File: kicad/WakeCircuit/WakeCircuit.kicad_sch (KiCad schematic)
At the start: 15 parts, among them J1 Conn_01x12_Socket, J2 Conn_01x10_Socket, U1 TLV7011DBVR, U3 4013

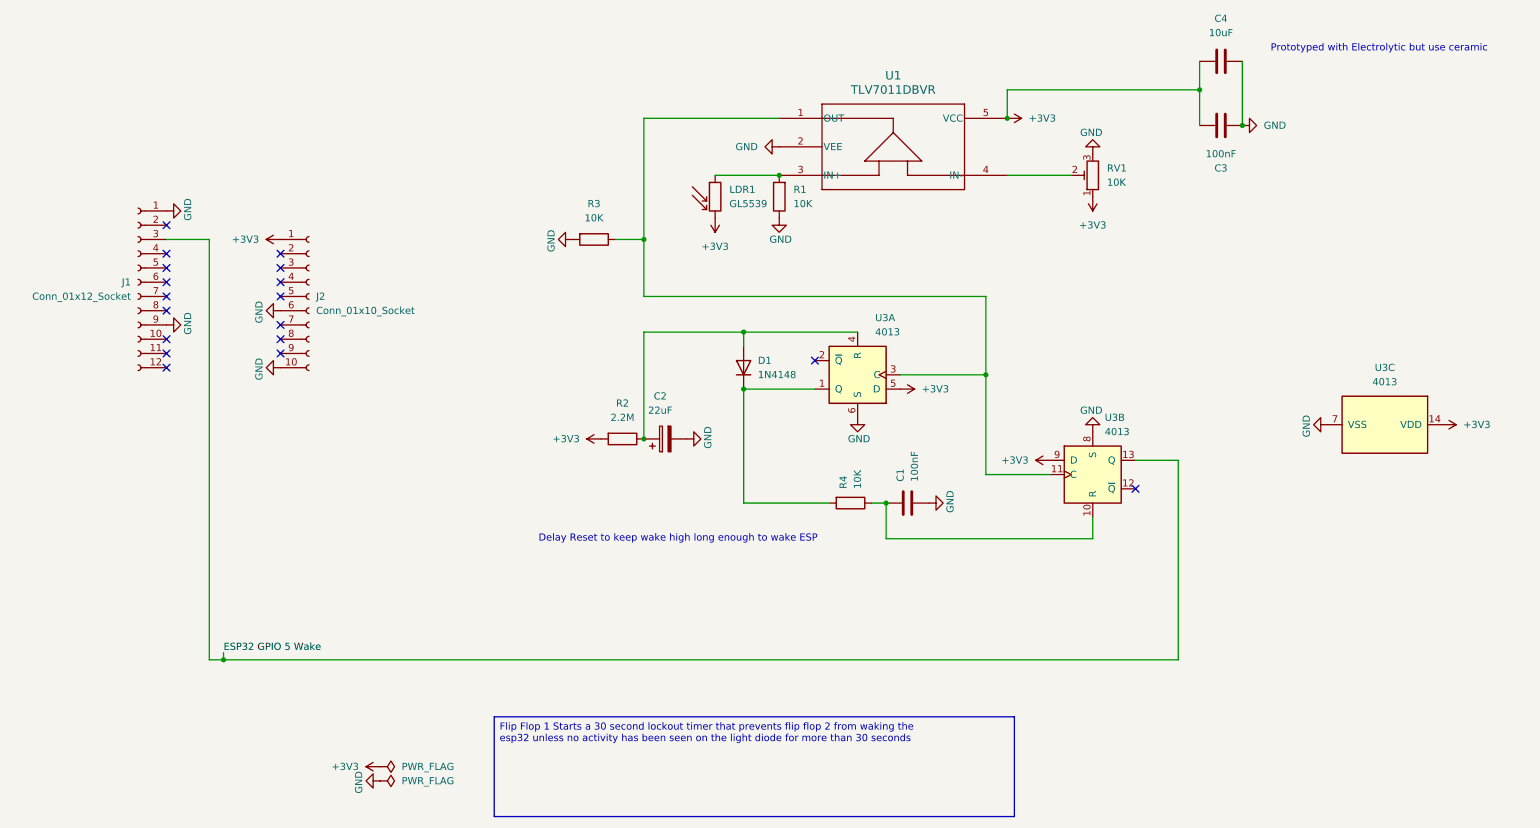
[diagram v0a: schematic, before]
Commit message: PCB layout
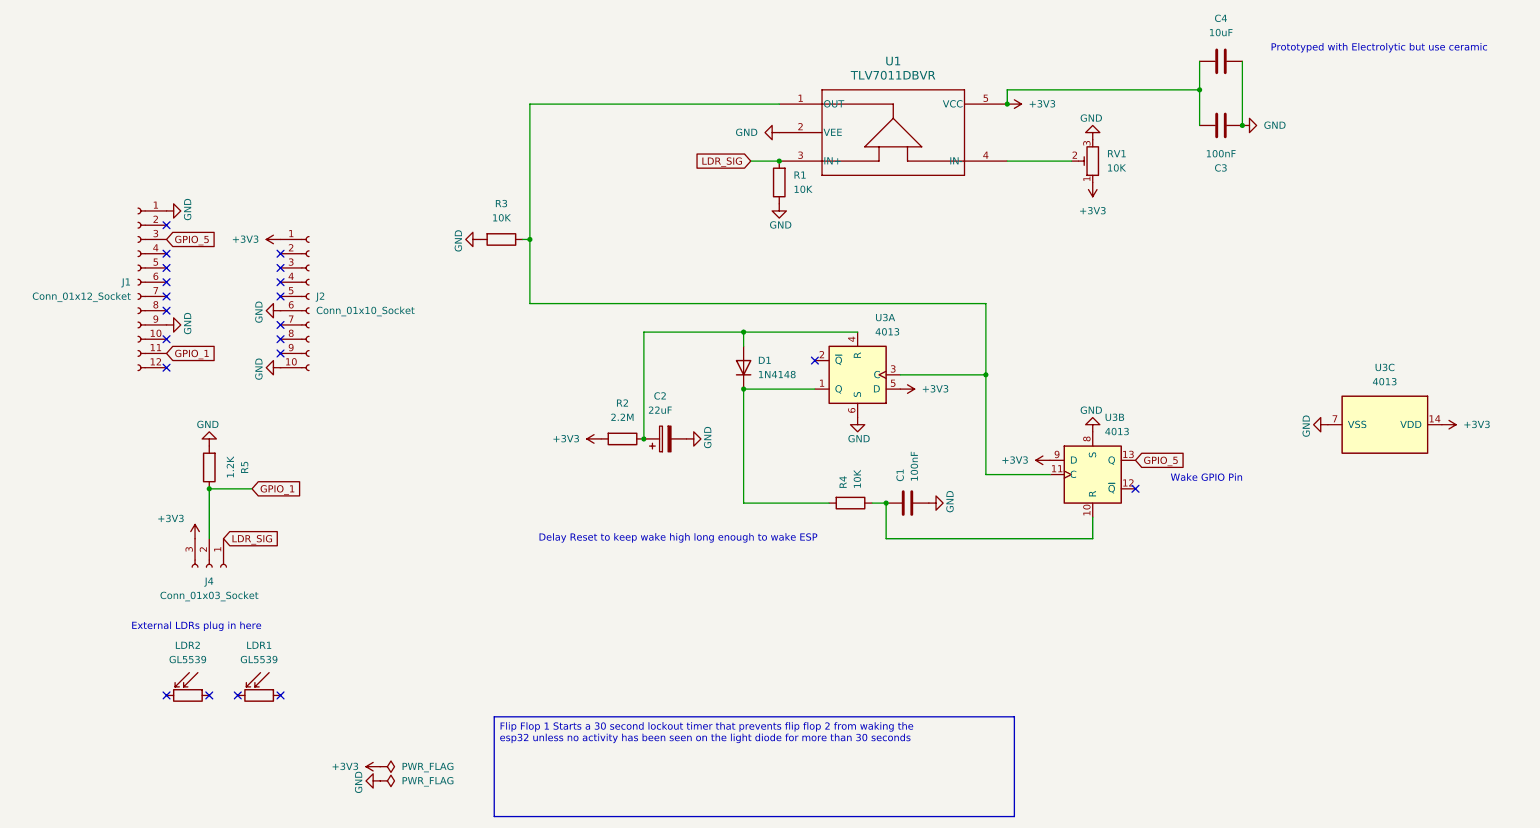
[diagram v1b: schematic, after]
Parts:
- added J4: Conn_01x03_Socket, Connector_JST:JST_PH_S3B-PH-K_1x03_P2.00mm_Horizontal, symbol Connector:Conn_01x03_Socket
- added LDR2: GL5539, OptoDevice:R_LDR_4.9x4.2mm_P2.54mm_Vertical, symbol Sensor_Optical:VT93xx
- added R5: 1.2K, Resistor_SMD:R_0805_2012Metric, symbol Device:R
- D1: footprint Diode_THT:D_DO-35_SOD27_P7.62mm_Horizontal -> Diode_SMD:D_SOD-123F
- RV1: footprint Potentiometer_THT:Potentiometer_Bourns_3386W_Horizontal -> Potentiometer_SMD:Potentiometer_Bourns_3214J_Horizontal
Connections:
- net +3V3: now also J4.3 (Pin_3); no longer LDR1.2
- net GND: now also R5.2
- net LDR_SIG: now reaches R1.2, U1.3 (IN+)
- net LDR_SIG: now also J4.1 (Pin_1); no longer LDR1.1
- net GPIO_1: now reaches J1.11 (Pin_11)
- net GPIO_1: now also J4.2 (Pin_2), R5.1
- net ESP32 GPIO 5 Wake renamed GPIO_5
- no-connect marks 18 -> 21
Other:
- note added: "External LDRs plug in here"
- note added: "Wake GPIO Pin"
- title: (none) -> M5Stamp C3 shield to wake on light detected
- moved on the sheet: R1, R3, RV1, U1
